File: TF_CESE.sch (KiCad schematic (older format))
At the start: 20 parts, among them IC1 SN74HC165N, IC2 SN74HC165N, J1 Conn_01x04, J2 Conn_01x03, J3 SD_Card, J4 Conn_01x08, J5 Conn_01x08, K1 SANYOU_SRD-05VDC-SL-C, Q1 2N2222A, Q2 S8050, U1 DHT11, U2 RC1602A

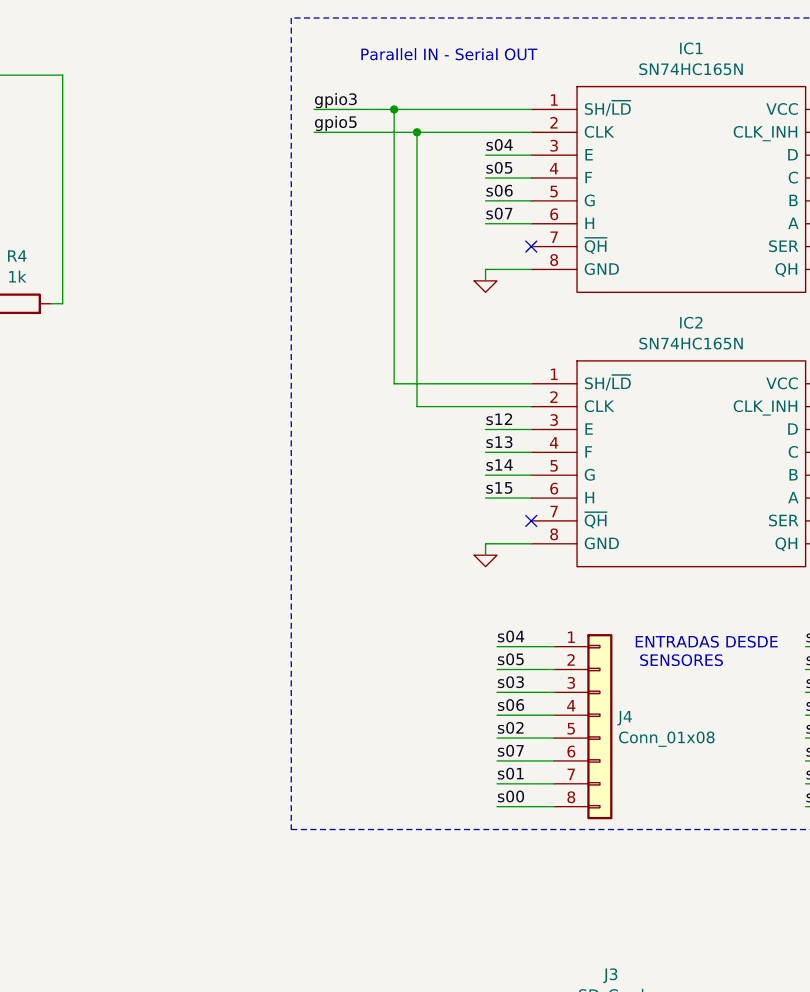
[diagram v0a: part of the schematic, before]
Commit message: Add files via upload
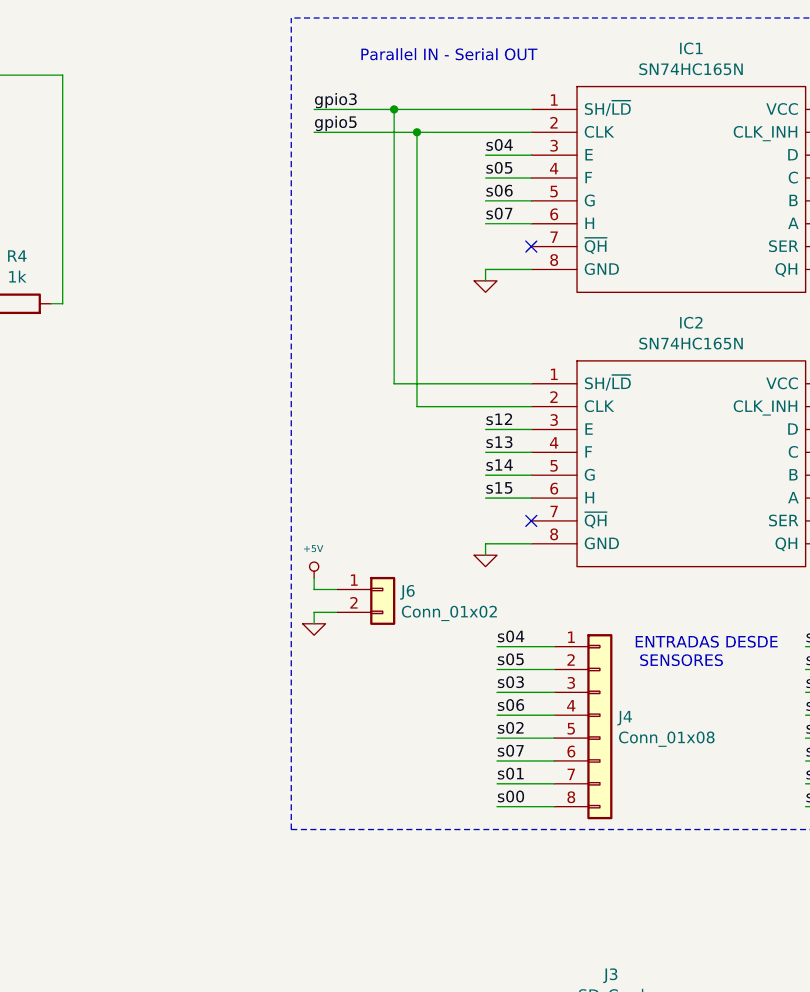
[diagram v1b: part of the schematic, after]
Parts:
- added J6: Conn_01x02, TerminalBlock_Phoenix:TerminalBlock_Phoenix_MKDS-1,5-2-5.08_1x02_P5.08mm_Horizontal, symbol Connector_Generic:Conn_01x02
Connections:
- net +5V: now also J6.1 (Pin_1)
- net GND: now also J6.2 (Pin_2)
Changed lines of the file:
@@
 	11050 650  7650 650
-Wire Notes Line
-	7650 650  7650 4200
 Wire Notes Line
 	7650 4200 11050 4200
@@
 	1650 1350 1650 1450
 $Comp
-L Misc_Poncho_Grande:GND #PWR?
+L Misc_Poncho_Grande:GND #PWR0101
 U 1 1 5F89E0BD
 P 3600 3400
-F 0 "#PWR?" H 3600 3400 30  0001 C CNN
+F 0 "#PWR0101" H 3600 3400 30  0001 C CNN
 F 1 "GND" H 3600 3330 30  0001 C CNN
 F 2 "" H 3600 3400 60  0000 C CNN
@@
 NoConn ~ 2400 2450
 NoConn ~ 2400 2550
+$Comp
+L Connector_Generic:Conn_01x02 J6
+U 1 1 5F7B509F
+P 8050 3150
+F 0 "J6" H 8130 3142 50  0000 L CNN
+F 1 "Conn_01x02" H 8130 3051 50  0000 L CNN
+F 2 "TerminalBlock_Phoenix:TerminalBlock_Phoenix_MKDS-1,5-2-5.08_1x02_P5.08mm_Horizontal" H 8050 3150 50  0001 C CNN
+F 3 "~" H 8050 3150 50  0001 C CNN
+	1    8050 3150
+	1    0    0    -1
+$EndComp
+$Comp
+L Misc_Poncho_Grande:GND #PWR0102
+U 1 1 5F7B80F3
+P 7750 3300
+F 0 "#PWR0102" H 7750 3300 30  0001 C CNN
+F 1 "GND" H 7750 3230 30  0001 C CNN
+F 2 "" H 7750 3300 60  0000 C CNN
+F 3 "" H 7750 3300 60  0000 C CNN
+	1    7750 3300
+	1    0    0    -1
+$EndComp
+Wire Wire Line
+	7750 3300 7750 3250
+$Comp
+L Misc_Poncho_Grande:+5V #PWR0103
+U 1 1 5F7C1247
+P 7750 3100
+F 0 "#PWR0103" H 7750 3190 20  0001 C CNN
+F 1 "+5V" H 7746 3228 30  0000 C CNN
+F 2 "" H 7750 3100 60  0000 C CNN
+F 3 "" H 7750 3100 60  0000 C CNN
+	1    7750 3100
+	1    0    0    -1
+$EndComp
+Wire Wire Line
+	7750 3100 7750 3150
+Wire Wire Line
+	7850 3150 7750 3150
+Wire Wire Line
+	7850 3250 7750 3250
+Wire Notes Line
+	7650 4200 7650 650
 $EndSCHEMATC

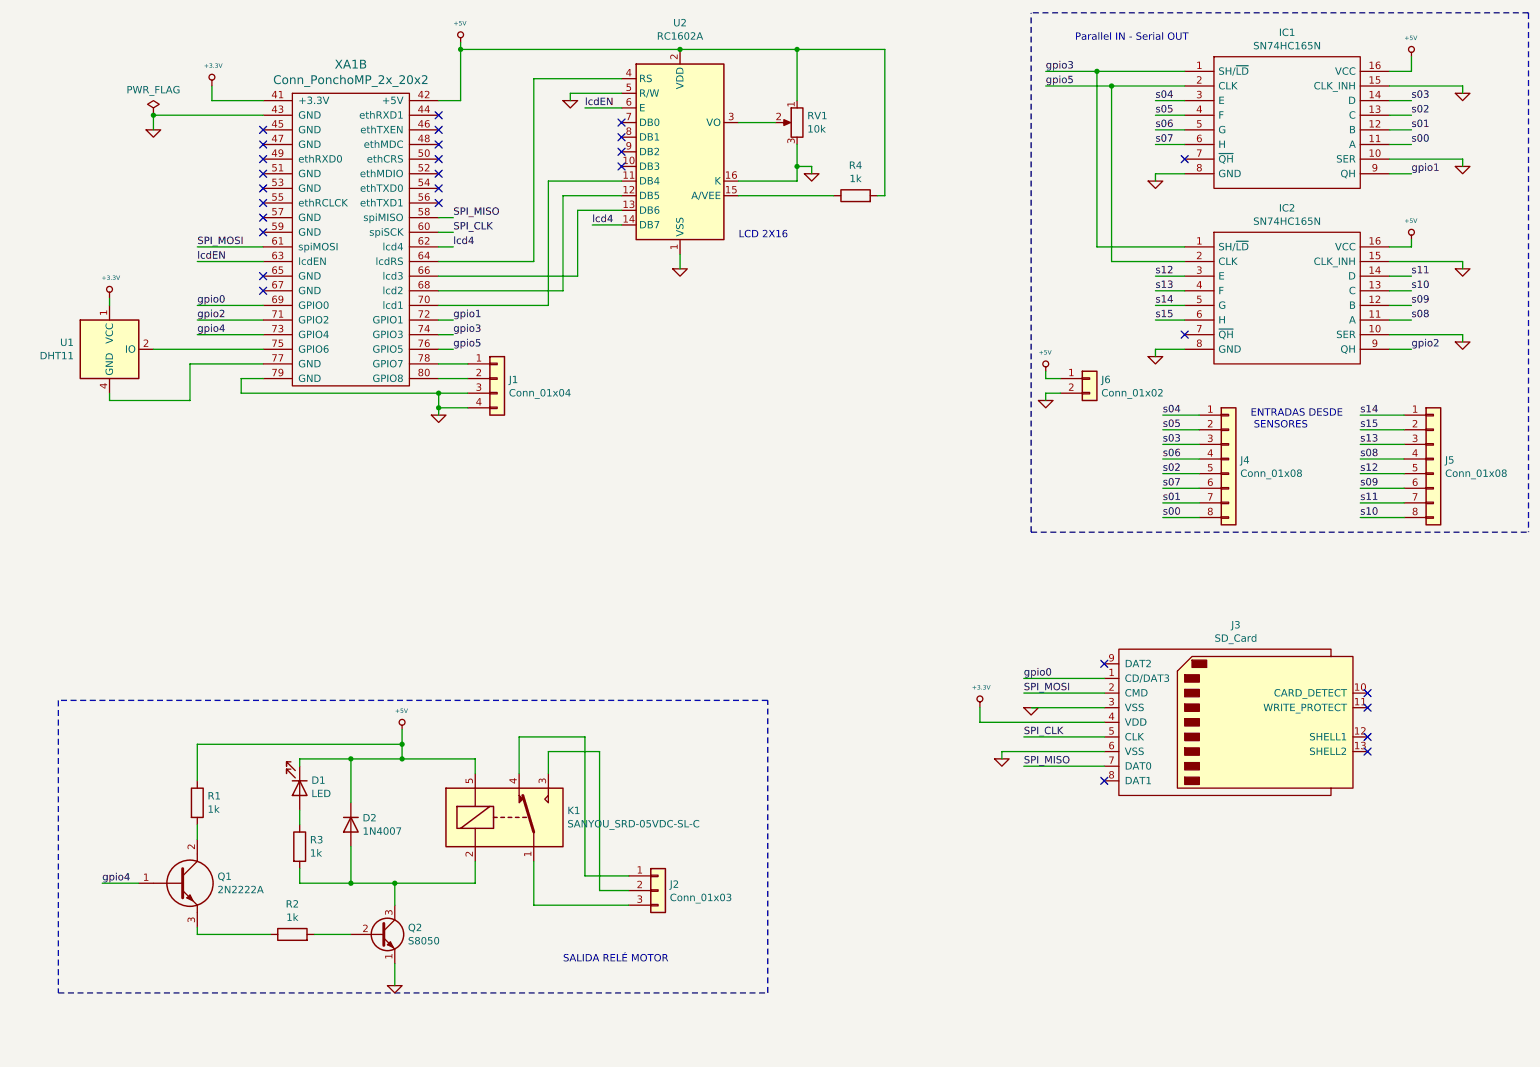
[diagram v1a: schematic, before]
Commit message: Add files via upload
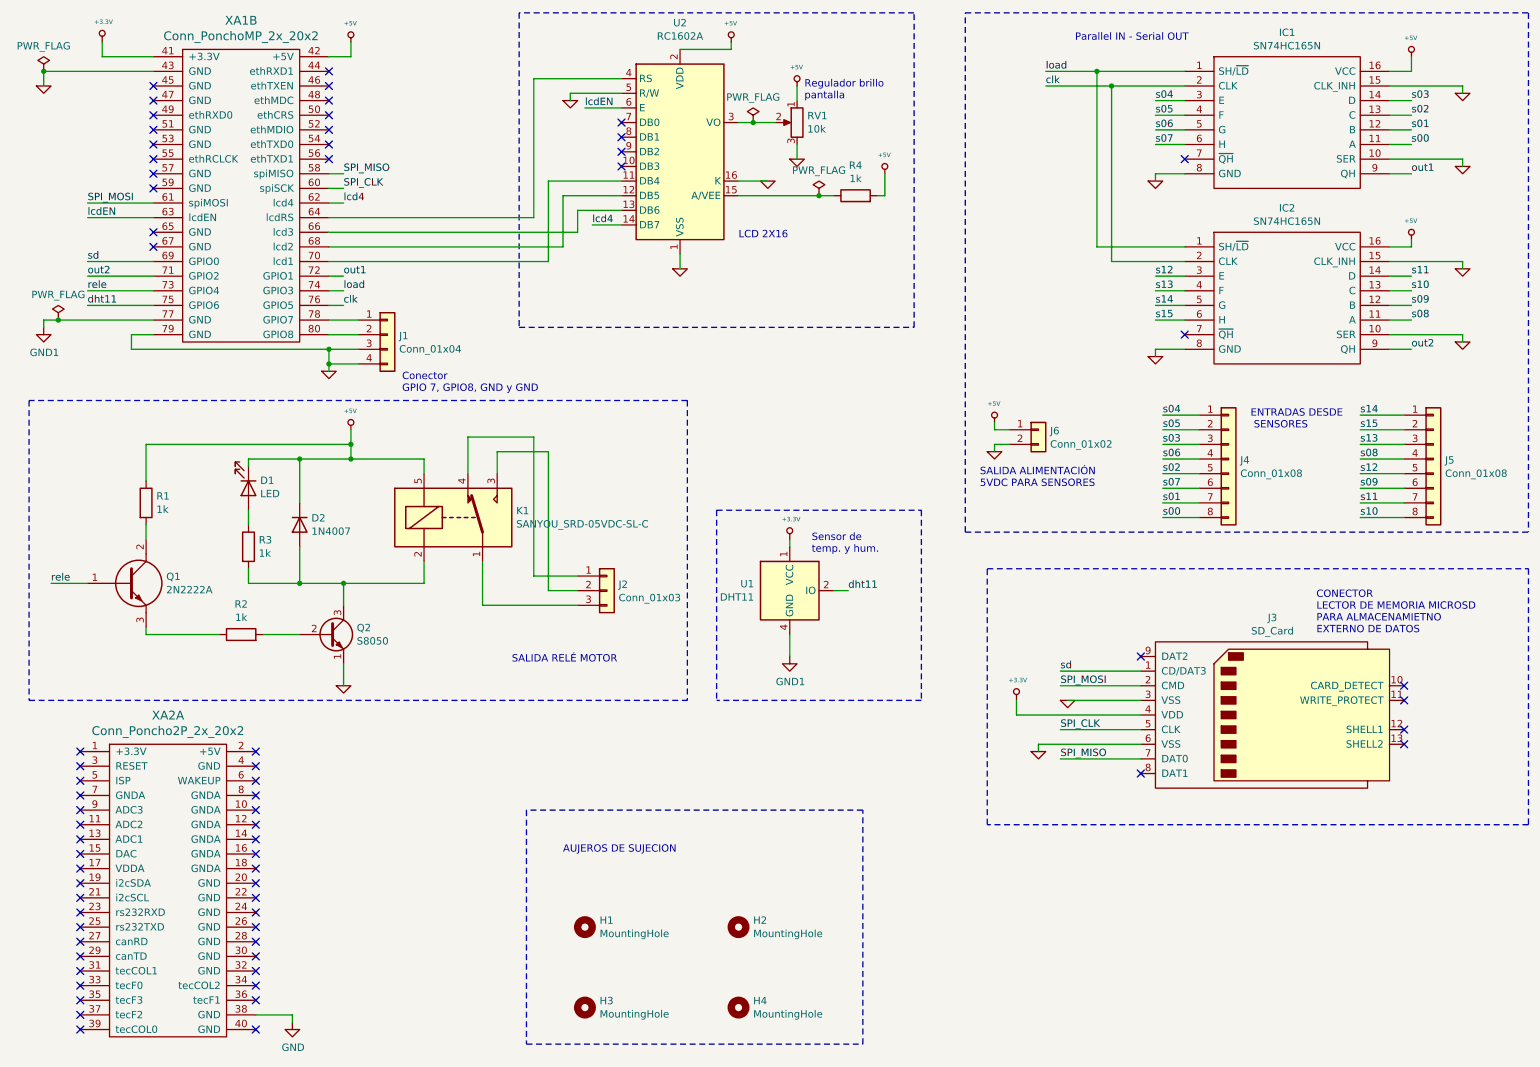
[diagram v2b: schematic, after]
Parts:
- added H1, H2: MountingHole, MountingHole:MountingHole_3.7mm, symbol Mechanical:MountingHole
- added H3: MountingHole, MountingHole:MountingHole_2.7mm, symbol Mechanical:MountingHole
- added H4: MountingHole, MountingHole:MountingHole_2.1mm, symbol Mechanical:MountingHole
- added XA2: Conn_Poncho2P_2x_20x2, Poncho_Esqueleto:Conn_Poncho_Derecha, symbol Poncho_Esqueleto:Conn_Poncho2P_2x_20x2
- IC1, IC2: footprint KiCad:DIP794W53P254L1930H508Q16N -> Package_DIP:DIP-18_W7.62mm_Socket_LongPads
- K1: Part numer (none) -> SRD-05VDC-SL-C
- Q2: Part number (none) -> S8050L-x-T92-B
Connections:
- net GND: now also XA2.38 (GND)
- net dht11: now reaches U1.2 (IO), XA1.75 (GPIO6)
- net GND1: now reaches U1.4 (GND), XA1.77 (GND)
- net gpio0 renamed sd
- net gpio1 renamed out1
- net gpio2 renamed out2
- net gpio3 renamed load
- net gpio4 renamed rele
- net gpio5 renamed clk
- no-connect marks 29 -> 68
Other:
- note added: "AUJEROS DE SUJECION"
- note added: "CONECTOR\nLECTOR DE MEMORIA MICROSD\nPARA ALMACENAMIETNO \nEXTERNO DE DATOS"
- note added: "Conector\nGPIO 7, GPIO8, GND y GND\n"
- note added: "Regulador brillo \npantalla"
- note added: "SALIDA ALIMENTACIÓN\n5VDC PARA SENSORES"
- note added: "Sensor de \ntemp. y hum."
- moved on the sheet: D1, D2, J1, J2, J3, J6, K1, Q1, Q2, R1, R2, R3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
